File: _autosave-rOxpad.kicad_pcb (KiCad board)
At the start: 2 copper layers, 77.8 x 63.5 mm, 22 parts, among them SW1 SW_Push, U1 ATmega32U4-A, Y1 16MHz

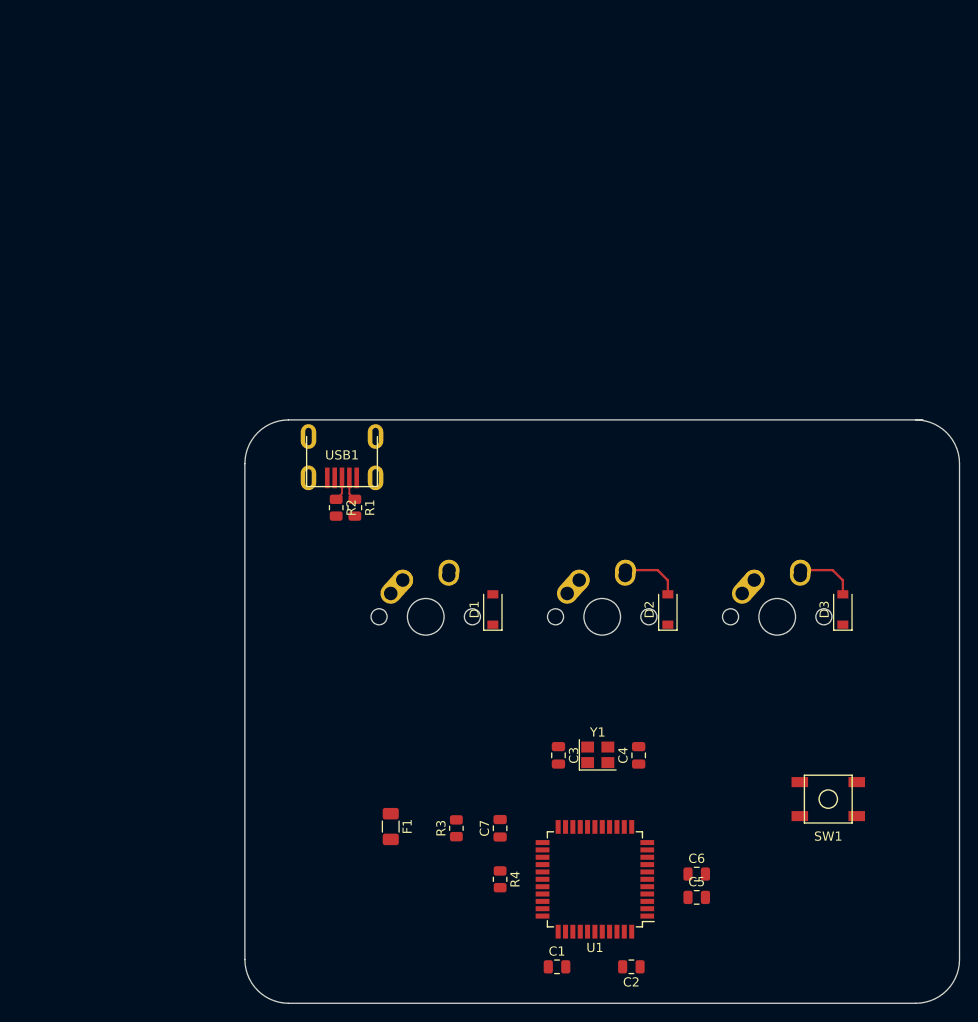
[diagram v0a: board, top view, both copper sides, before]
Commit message: I think the pcb is done wohoo
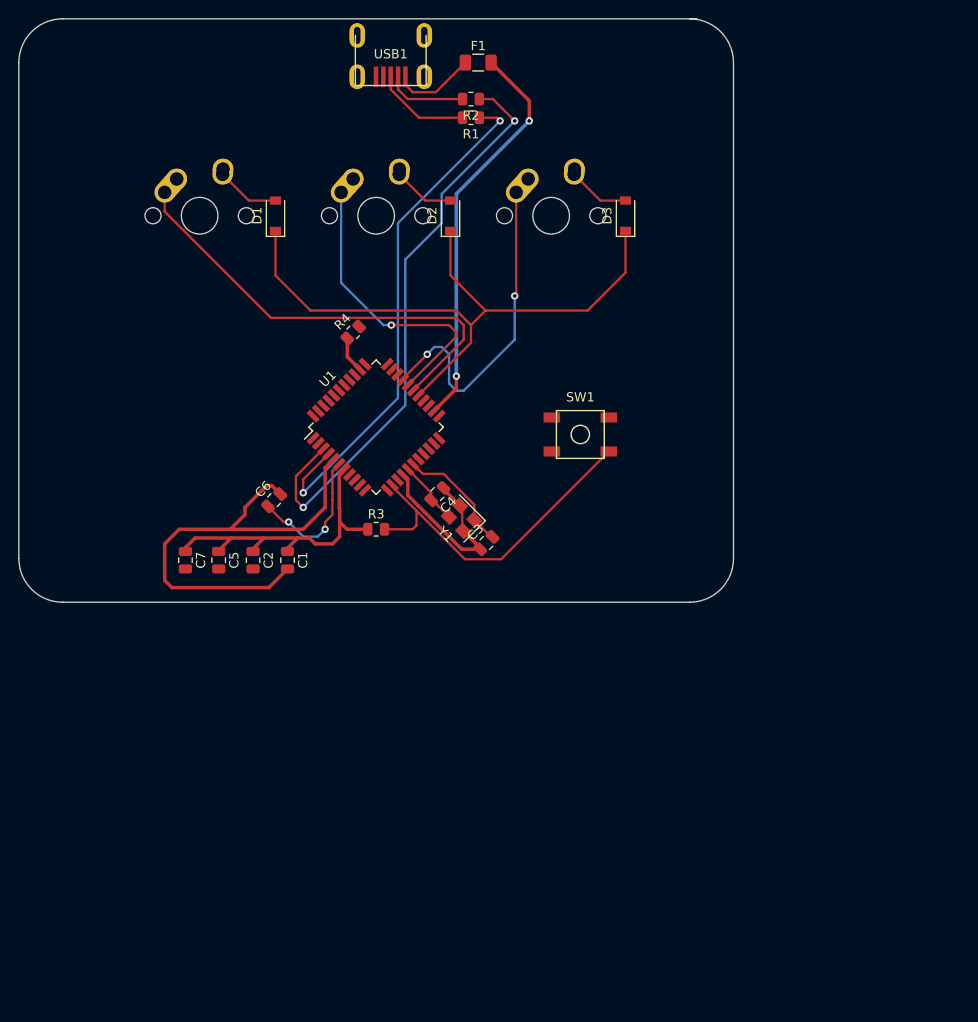
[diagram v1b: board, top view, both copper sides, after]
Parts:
- moved F1 83.7 mm to (107.2, 52.4), turned to 0 degrees
- moved C5 63.7 mm to (78.9, 106.6), turned to -90 degrees
- moved R4 61.6 mm to (93.5, 81.8), turned to 45 degrees
- moved C6 61.4 mm to (84.9, 100.0), turned to 45 degrees
- moved C2 60.5 mm to (82.6, 106.6), turned to -90 degrees
- moved U1 54.7 mm to (96.0, 92.1), turned to 45 degrees
- moved C1 53.1 mm to (86.4, 106.6), turned to -90 degrees
- moved MX1 50.1 mm to (76.8, 69.1)
- moved MX2 50.1 mm to (96.0, 69.1)
- moved MX3 50.1 mm to (115.1, 69.1)
- moved D1 49.0 mm to (85.1, 69.1)
- moved D2 49.0 mm to (104.1, 69.1)
- moved D3 49.0 mm to (123.2, 69.1)
- moved SW1 48.0 mm to (118.3, 92.9), turned to 180 degrees
- moved R1 46.2 mm to (106.4, 56.4), turned to 0 degrees
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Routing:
- net +5V: track 0.48 -> 79.0 mm, vias 0 -> 2
- net GND: track 0.61 -> 76.6 mm
- net ROW-0: track 0.00 -> 72.4 mm
- net Net-(R1-Pad2): track 0.00 -> 64.4 mm, vias 0 -> 2
- net Net-(R2-Pad2): track 0.00 -> 57.2 mm, vias 0 -> 2
- net COL-0: track 0.00 -> 49.1 mm
- net Net-(R3-Pad2): track 0.00 -> 37.1 mm
- net COL-2: track 0.00 -> 36.0 mm, vias 0 -> 2
- net COL-1: track 0.00 -> 32.5 mm, vias 0 -> 1
- net Net-(C6-Pad1): track 0.00 -> 15.6 mm, vias 0 -> 2
- net Net-(C3-Pad2): track 0.22 -> 12.9 mm
- net Net-(F1-Pad1): track 0.00 -> 9.07 mm
- net D+: track 2.60 -> 10.5 mm
- net Net-(D1-Pad2): track 0.00 -> 6.94 mm
- net Net-(C4-Pad2): track 0.56 -> 7.08 mm
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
